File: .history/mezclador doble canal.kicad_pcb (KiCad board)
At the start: 2 copper layers, 53.4 x 51.5 mm, 45 parts, among them J1 Conn_Coaxial, J2 Conn_Coaxial, J3 Conn_Coaxial, J4 Conn_Coaxial, J5 Conn_Coaxial, J6 Conn_Coaxial, J7 Screw_Terminal_01x02, J8 Conn_Coaxial, SW1 SW_SPST, U1 NE5532, U2 TL071

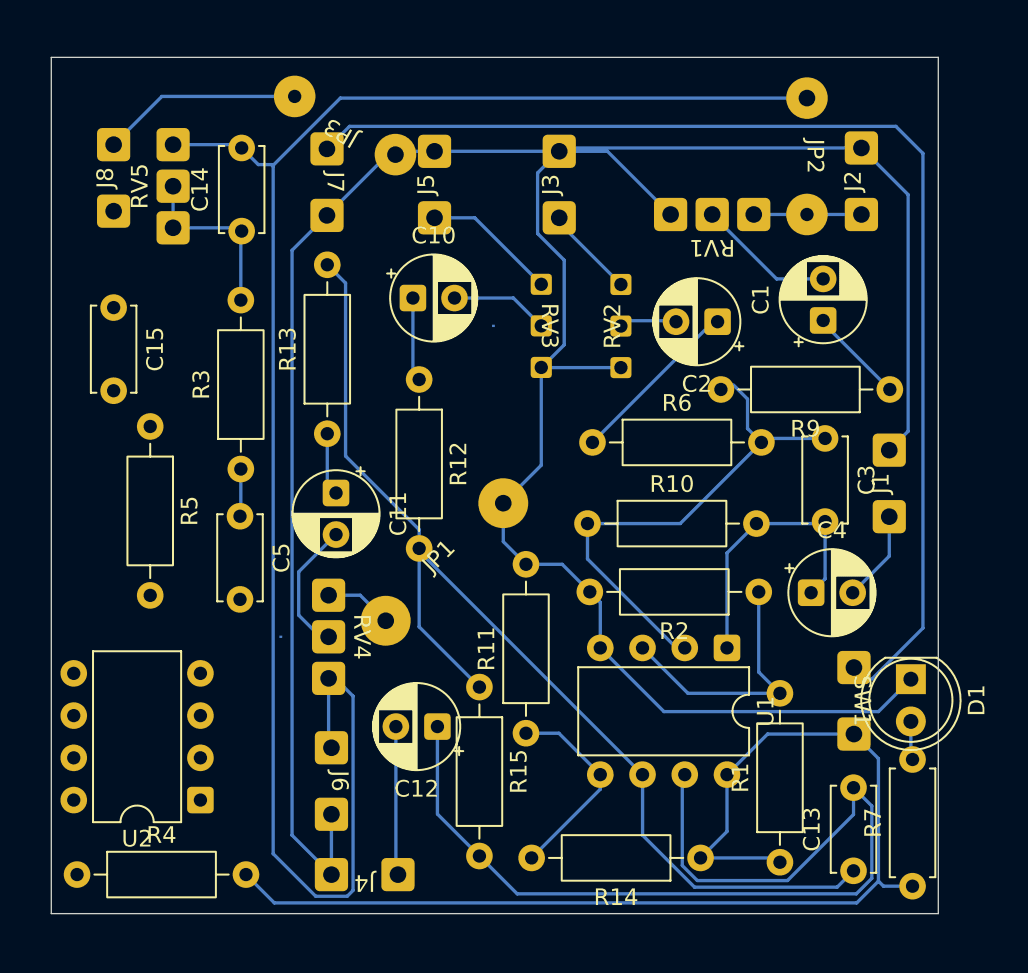
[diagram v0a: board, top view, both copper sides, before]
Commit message: todos los componentes enrutadosgit add .!
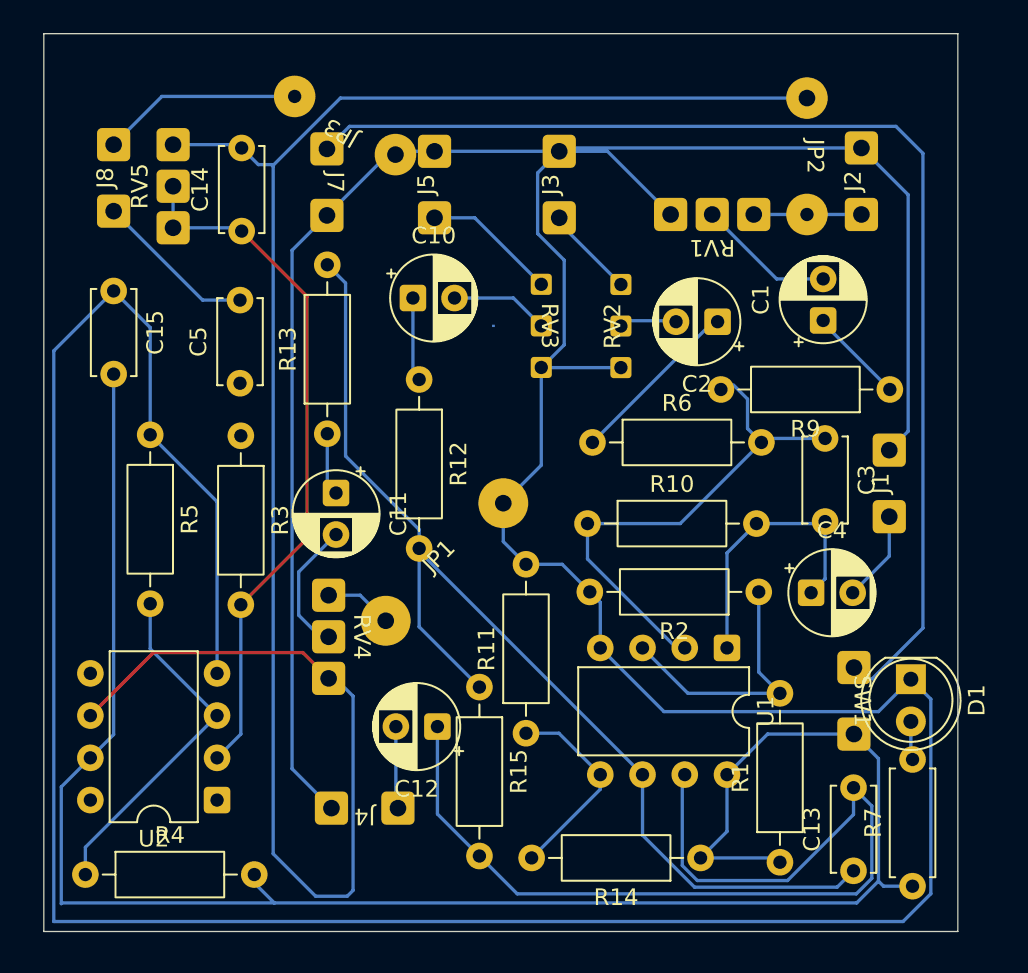
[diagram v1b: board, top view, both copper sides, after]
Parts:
- removed J6: Conn_Coaxial, personal:double wire
- moved C5 8.00 mm to (171.3, 62.0), turned to 90 degrees
- moved J4 4.00 mm to (178.8, 87.5)
- moved R3 2.00 mm to (171.3, 65.1), turned to -90 degrees
- moved C15 1.00 mm to (163.7, 56.4)
- moved U2 1.00 mm to (169.9, 87.0)
- moved R4 0.50 mm to (162.0, 91.5)
- moved R5 0.50 mm to (165.9, 65.0)
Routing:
- net GND: track 170.4 -> 294.6 mm
- net VCC: track 70.1 -> 116.1 mm
- net Net-(U2--): track 10.9 -> 42.5 mm
- net Net-(U2-+): track 0.00 -> 21.2 mm
- net Net-(JP2-A): track 101.0 -> 117.5 mm
- net Net-(J8-In): track 0.00 -> 9.82 mm
- net Net-(J6-In): track 4.25 -> 0.00 mm
- net Net-(J4-In): track 8.96 -> 4.96 mm
- net Net-(C5-Pad1): track 2.86 -> 0.00 mm
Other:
- board size 53.4 x 51.5 mm -> 55 x 54 mm

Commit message: todo en su lugar / tamaño 50x55
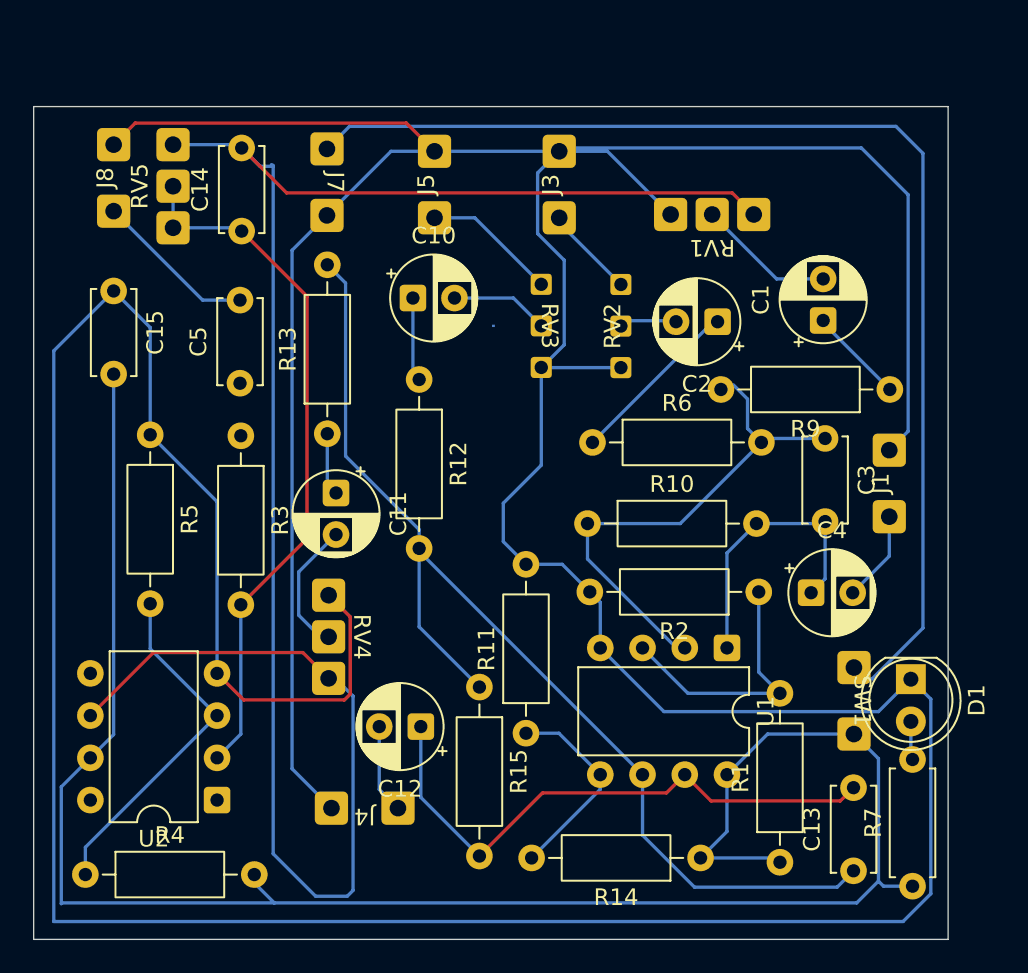
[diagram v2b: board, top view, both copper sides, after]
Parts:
- removed J2: Conn_Coaxial, personal:double wire
- removed JP1: Jumper_2_Bridged, personal:Jumper_Wire_10mm
- removed JP2, JP3: Jumper_2_Bridged, personal:Jumper_Wire_7mm
- moved C12 1.00 mm to (182.2, 82.6)
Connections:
- C14 pad 2: Net-(JP2-A) -> Net-(C14-Pad2)
- J8 pad 2: Net-(J8-Ext) -> GND
- RV1 pad 1: Net-(JP2-B) -> Net-(C14-Pad2)
- RV4 pad 1: Net-(JP1-A) -> GND
- RV4 pad 3: Net-(JP2-A) -> Net-(C14-Pad2)
- RV5 pad 3: Net-(JP2-A) -> Net-(C14-Pad2)
- U2 pad 6: Net-(JP2-A) -> Net-(C14-Pad2)
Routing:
- net Net-(JP2-A): track 117.5 -> 0.00 mm
- net Net-(C14-Pad2): track 0.00 -> 116.5 mm
- net GND: track 294.6 -> 330.7 mm
- net Net-(C12-Pad1): track 59.1 -> 35.0 mm
- net Net-(J8-Ext): track 12.1 -> 0.00 mm
- net Net-(J2-In): track 6.48 -> 0.00 mm
- net Net-(JP1-A): track 4.32 -> 0.00 mm
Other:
- board size 55 x 54 mm -> 55 x 50.1 mm
